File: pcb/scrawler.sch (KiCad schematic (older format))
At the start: 54 parts, among them SW1 switch, SW10 switch, SW11 switch, SW12 switch, SW13 switch, SW14 switch, SW15 switch, SW16 switch, SW17 switch, SW18 switch, SW19 switch, SW2 switch, SW20 switch, SW21 switch, SW22 switch, SW23 switch, SW3 switch, SW4 switch, SW5 switch, SW6 switch, SW7 switch, SW8 switch, SW9 switch, U1 TRRS, U2 ProMicro

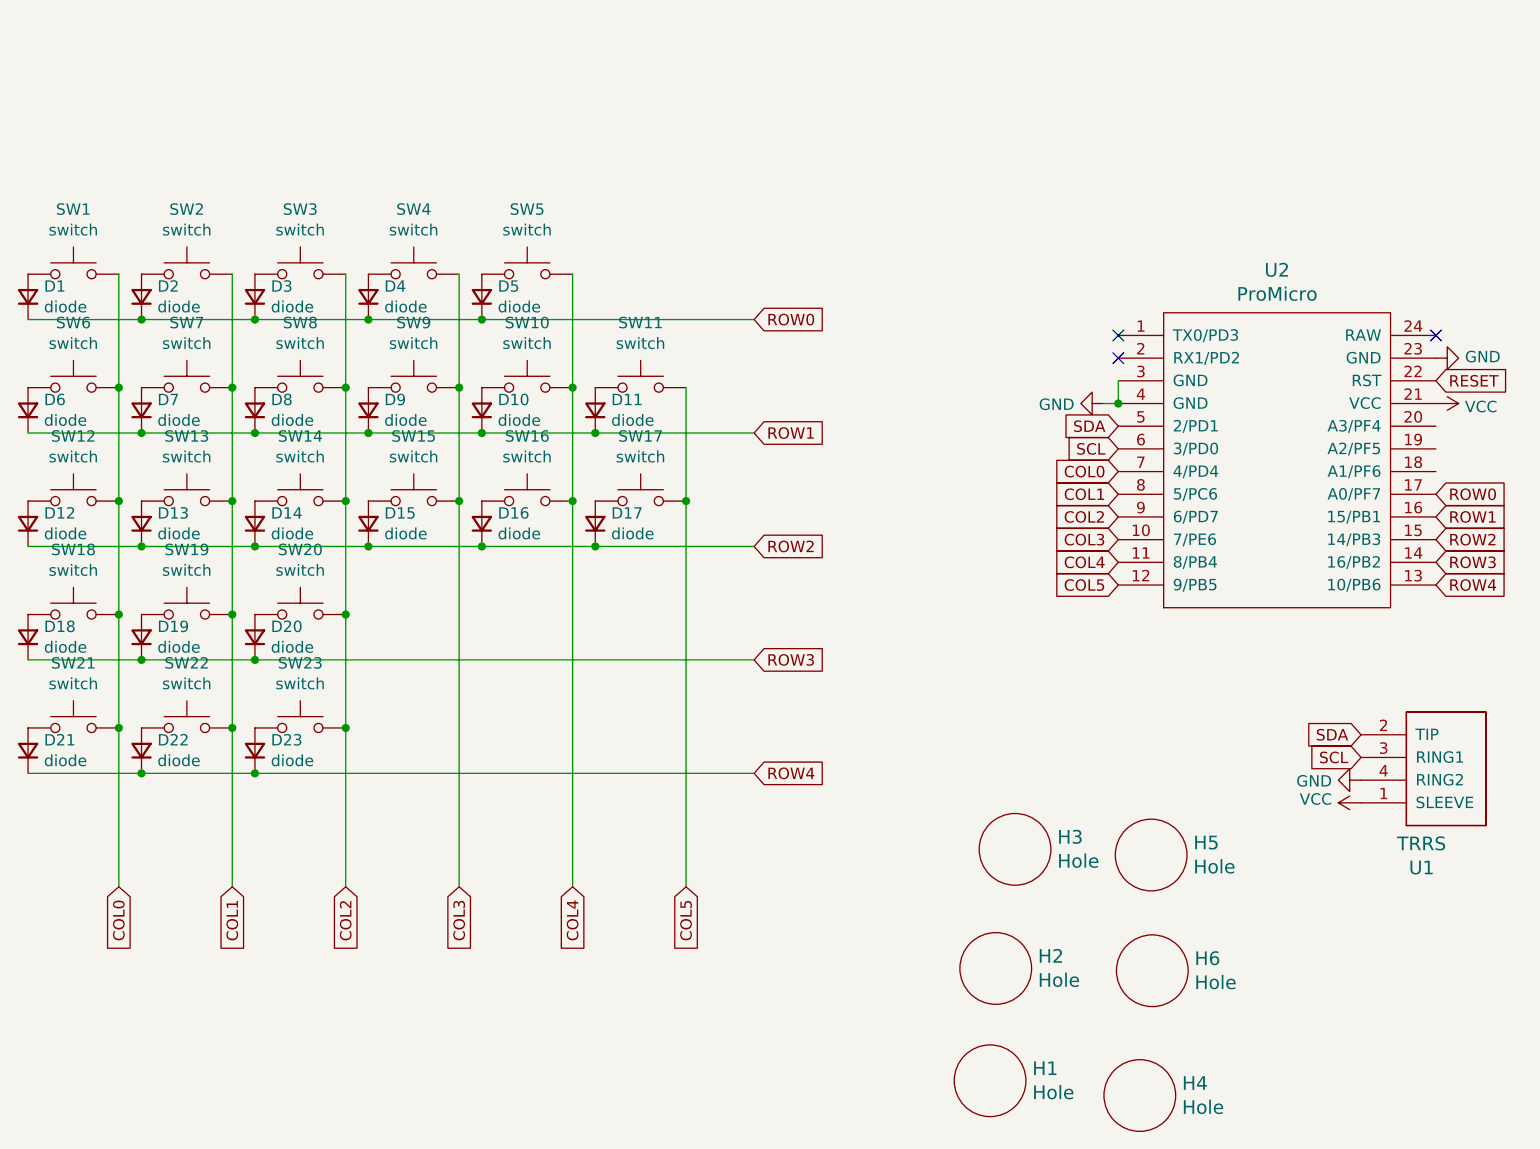
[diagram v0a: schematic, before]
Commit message: clean root dir
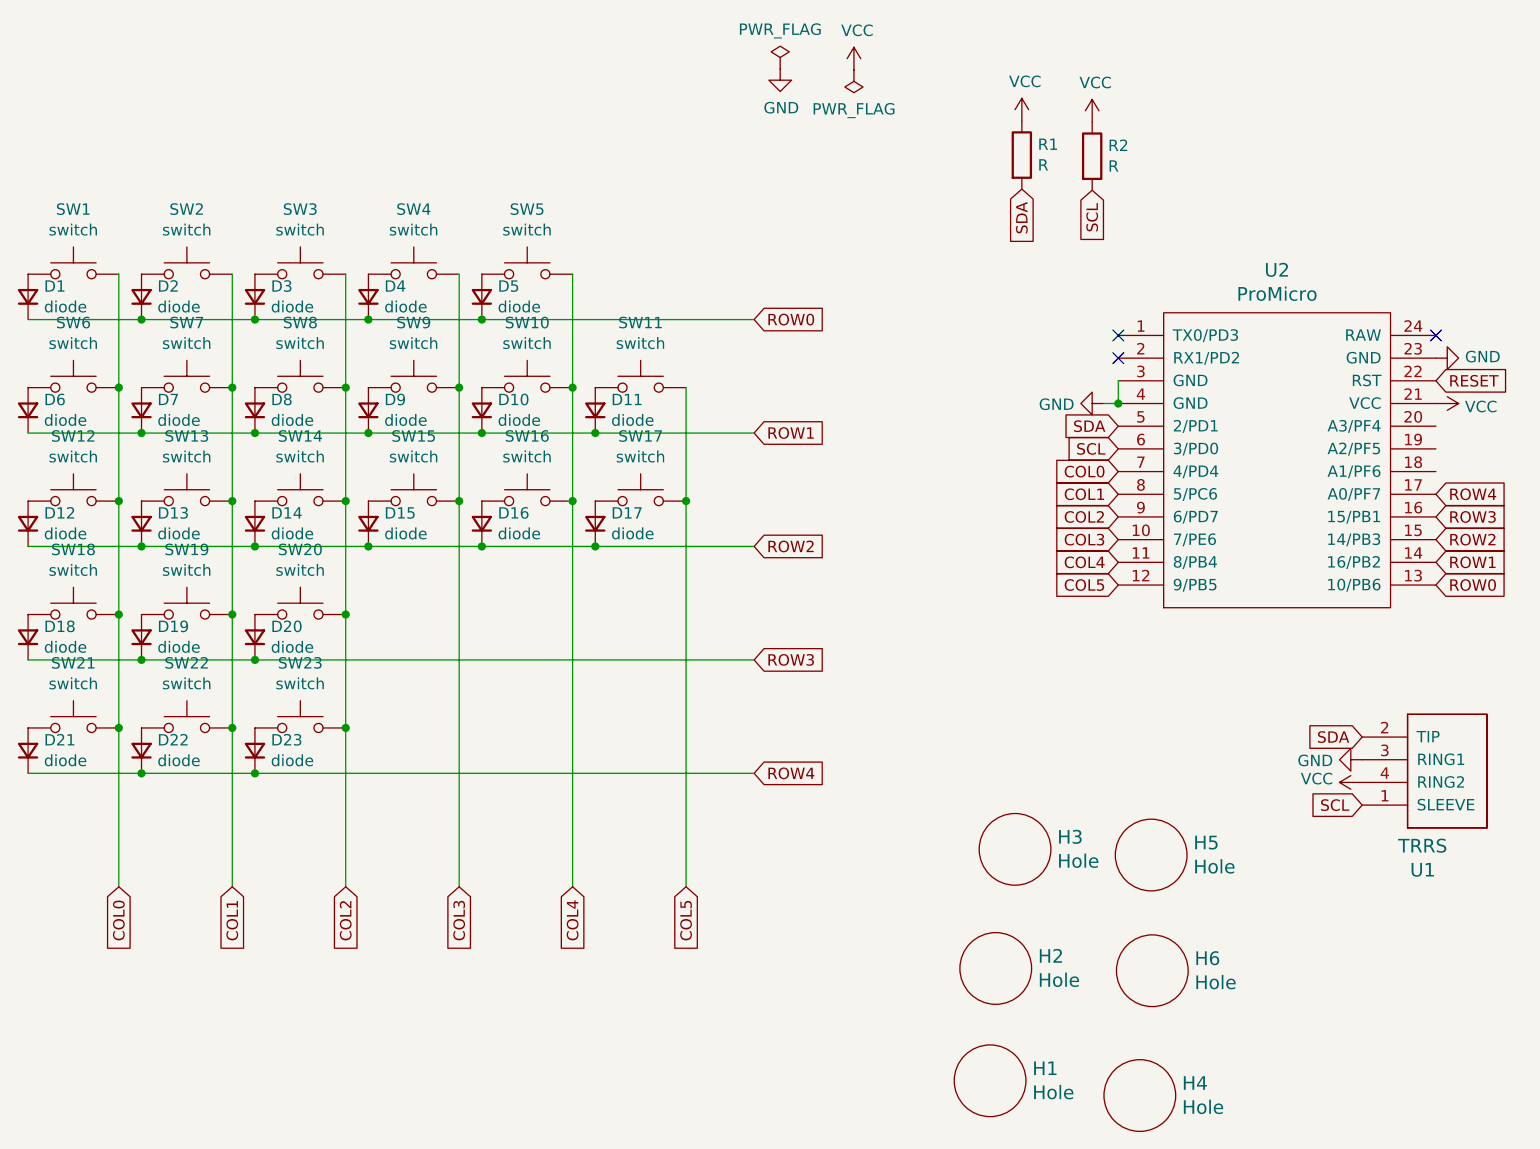
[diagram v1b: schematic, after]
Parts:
- added R1, R2: R, Keebio-Parts:Resistor, symbol Device:R
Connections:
- net GND: now also U1.3 (RING1); no longer U1.4 (RING2)
- net ROW0: now also U2.13 (10/PB6); no longer U2.17 (A0/PF7)
- net ROW1: now also U2.14 (16/PB2); no longer U2.16 (15/PB1)
- net ROW3: now also U2.16 (15/PB1); no longer U2.14 (16/PB2)
- net ROW4: now also U2.17 (A0/PF7); no longer U2.13 (10/PB6)
- net SCL: now also U1.1 (SLEEVE), R2.2; no longer U1.3 (RING1)
- net SDA: now also R1.2
- net VCC: now also U1.4 (RING2), R1.1, R2.1; no longer U1.1 (SLEEVE)
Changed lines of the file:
@@
 L keebio:TRRS U1
 U 1 1 60A4975E
-P 8075 4690
-F 0 "U1" H 7992 4503 60  0000 C CNN
-F 1 "TRRS" H 7992 4609 60  0000 C CNN
-F 2 "Keebio-Parts:TRRS-PJ-320A-dual" H 8225 4690 60  0001 C CNN
-F 3 "" H 8225 4690 60  0001 C CNN
-	1    8075 4690
+P 8080 4700
+F 0 "U1" H 7997 4513 60  0000 C CNN
+F 1 "TRRS" H 7997 4619 60  0000 C CNN
+F 2 "Keebio-Parts:TRRS-PJ-320A-dual" H 8230 4700 60  0001 C CNN
+F 3 "" H 8230 4700 60  0001 C CNN
+	1    8080 4700
 	1    0    0    -1
 $EndComp
@@
 Text GLabel 6655 3630 0    50   Input ~ 0
 COL5
-Text GLabel 8055 3230 2    50   Input ~ 0
+Text GLabel 8055 3630 2    50   Input ~ 0
 ROW0
-Text GLabel 8055 3330 2    50   Input ~ 0
+Text GLabel 8055 3530 2    50   Input ~ 0
 ROW1
 Text GLabel 8055 3430 2    50   Input ~ 0
 ROW2
-Text GLabel 8055 3530 2    50   Input ~ 0
+Text GLabel 8055 3330 2    50   Input ~ 0
 ROW3
-Text GLabel 8055 3630 2    50   Input ~ 0
+Text GLabel 8055 3230 2    50   Input ~ 0
 ROW4
 Text GLabel 8055 2730 2    50   Input ~ 0
@@
 L power:VCC #PWR0104
 U 1 1 60A698CA
-P 7725 4590
-F 0 "#PWR0104" H 7725 4440 50  0001 C CNN
-F 1 "VCC" V 7740 4718 50  0000 L CNN
-F 2 "" H 7725 4590 50  0001 C CNN
-F 3 "" H 7725 4590 50  0001 C CNN
-	1    7725 4590
+P 7730 4500
+F 0 "#PWR0104" H 7730 4350 50  0001 C CNN
+F 1 "VCC" V 7745 4628 50  0000 L CNN
+F 2 "" H 7730 4500 50  0001 C CNN
+F 3 "" H 7730 4500 50  0001 C CNN
+	1    7730 4500
 	0    -1   -1   0
 $EndComp
@@
 L power:GND #PWR0105
 U 1 1 60A6A41D
-P 7725 4490
-F 0 "#PWR0105" H 7725 4240 50  0001 C CNN
-F 1 "GND" V 7730 4362 50  0000 R CNN
-F 2 "" H 7725 4490 50  0001 C CNN
-F 3 "" H 7725 4490 50  0001 C CNN
-	1    7725 4490
+P 7730 4400
+F 0 "#PWR0105" H 7730 4150 50  0001 C CNN
+F 1 "GND" V 7735 4272 50  0000 R CNN
+F 2 "" H 7730 4400 50  0001 C CNN
+F 3 "" H 7730 4400 50  0001 C CNN
+	1    7730 4400
 	0    1    1    0
 $EndComp
-Text GLabel 7725 4290 0    50   Input ~ 0
+Text GLabel 7730 4300 0    50   Input ~ 0
 SDA
-Text GLabel 7725 4390 0    50   Input ~ 0
+Text GLabel 7730 4600 0    50   Input ~ 0
 SCL
 $Comp
@@
 	1    0    0    -1
 $EndComp
+$Comp
+L Device:R R1
+U 1 1 60C01C38
+P 6230 1735
+F 0 "R1" H 6300 1781 50  0000 L CNN
+F 1 "R" H 6300 1690 50  0000 L CNN
+F 2 "Keebio-Parts:Resistor" V 6160 1735 50  0001 C CNN
+F 3 "~" H 6230 1735 50  0001 C CNN
+	1    6230 1735
+	1    0    0    -1
+$EndComp
+$Comp
+L Device:R R2
+U 1 1 60C0241A
+P 6540 1740
+F 0 "R2" H 6610 1786 50  0000 L CNN
+F 1 "R" H 6610 1695 50  0000 L CNN
+F 2 "Keebio-Parts:Resistor" V 6470 1740 50  0001 C CNN
+F 3 "~" H 6540 1740 50  0001 C CNN
+	1    6540 1740
+	1    0    0    -1
+$EndComp
+$Comp
+L power:VCC #PWR0106
+U 1 1 60C03FE0
+P 6230 1585
+F 0 "#PWR0106" H 6230 1435 50  0001 C CNN
+F 1 "VCC" H 6245 1758 50  0000 C CNN
+F 2 "" H 6230 1585 50  0001 C CNN
+F 3 "" H 6230 1585 50  0001 C CNN
+	1    6230 1585
+	1    0    0    -1
+$EndComp
+$Comp
+L power:VCC #PWR0107
+U 1 1 60C047F7
+P 6540 1590
+F 0 "#PWR0107" H 6540 1440 50  0001 C CNN
+F 1 "VCC" H 6555 1763 50  0000 C CNN
+F 2 "" H 6540 1590 50  0001 C CNN
+F 3 "" H 6540 1590 50  0001 C CNN
+	1    6540 1590
+	1    0    0    -1
+$EndComp
+Text GLabel 6230 1885 3    50   Input ~ 0
+SDA
+Text GLabel 6540 1890 3    50   Input ~ 0
+SCL
+$Comp
+L power:PWR_FLAG #FLG0101
+U 1 1 60C068F4
+P 5165 1355
+F 0 "#FLG0101" H 5165 1430 50  0001 C CNN
+F 1 "PWR_FLAG" H 5165 1528 50  0000 C CNN
+F 2 "" H 5165 1355 50  0001 C CNN
+F 3 "~" H 5165 1355 50  0001 C CNN
+	1    5165 1355
+	1    0    0    -1
+$EndComp
+$Comp
+L power:GND #PWR0108
+U 1 1 60C073E6
+P 5165 1355
+F 0 "#PWR0108" H 5165 1105 50  0001 C CNN
+F 1 "GND" H 5170 1182 50  0000 C CNN
+F 2 "" H 5165 1355 50  0001 C CNN
+F 3 "" H 5165 1355 50  0001 C CNN
+	1    5165 1355
+	1    0    0    -1
+$EndComp
+$Comp
+L power:PWR_FLAG #FLG0102
+U 1 1 60C07A4D
+P 5490 1360
+F 0 "#FLG0102" H 5490 1435 50  0001 C CNN
+F 1 "PWR_FLAG" H 5490 1533 50  0000 C CNN
+F 2 "" H 5490 1360 50  0001 C CNN
+F 3 "~" H 5490 1360 50  0001 C CNN
+	1    5490 1360
+	-1   0    0    1
+$EndComp
+$Comp
+L power:VCC #PWR0109
+U 1 1 60C0818C
+P 5490 1360
+F 0 "#PWR0109" H 5490 1210 50  0001 C CNN
+F 1 "VCC" H 5505 1533 50  0000 C CNN
+F 2 "" H 5490 1360 50  0001 C CNN
+F 3 "" H 5490 1360 50  0001 C CNN
+	1    5490 1360
+	1    0    0    -1
+$EndComp
